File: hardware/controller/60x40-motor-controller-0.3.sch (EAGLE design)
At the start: 19 parts, among them IC1 TS432A-A3G, IC2 TS432A-A3G

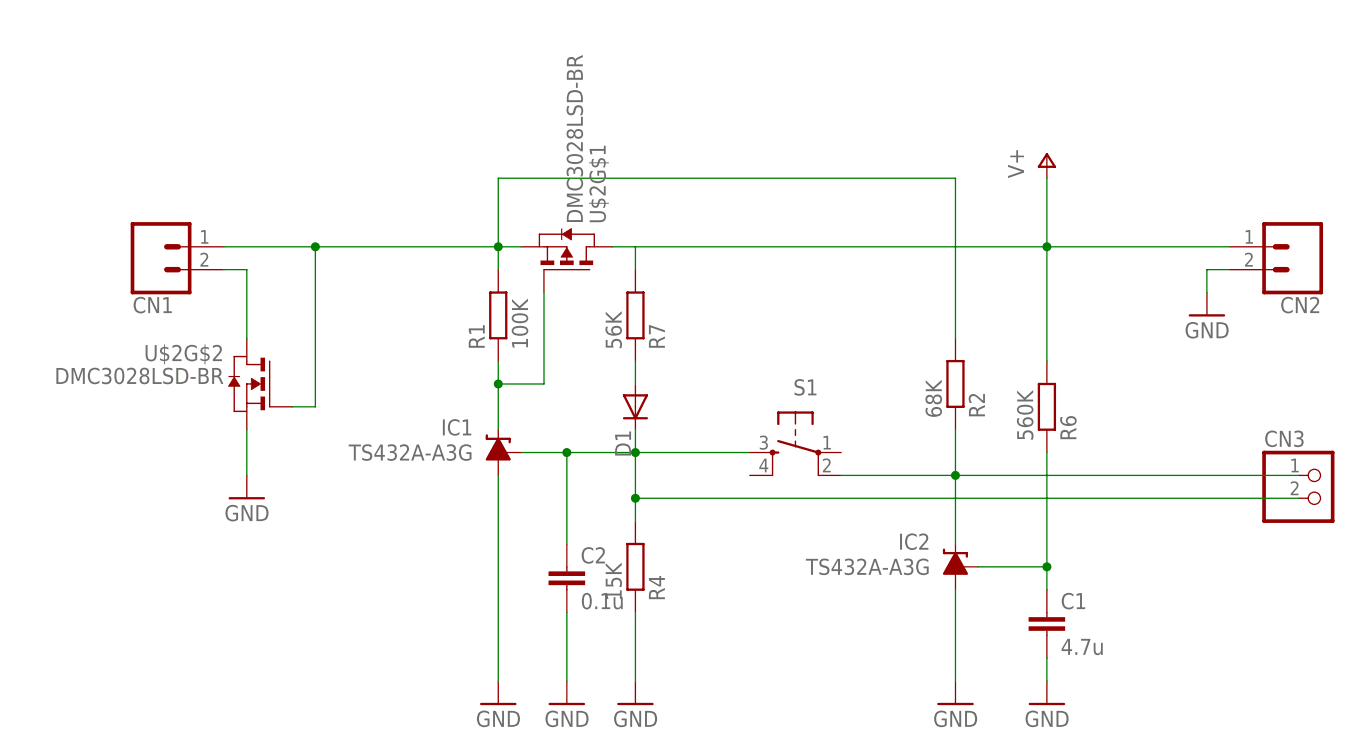
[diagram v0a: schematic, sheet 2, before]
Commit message: Lots of controller designs
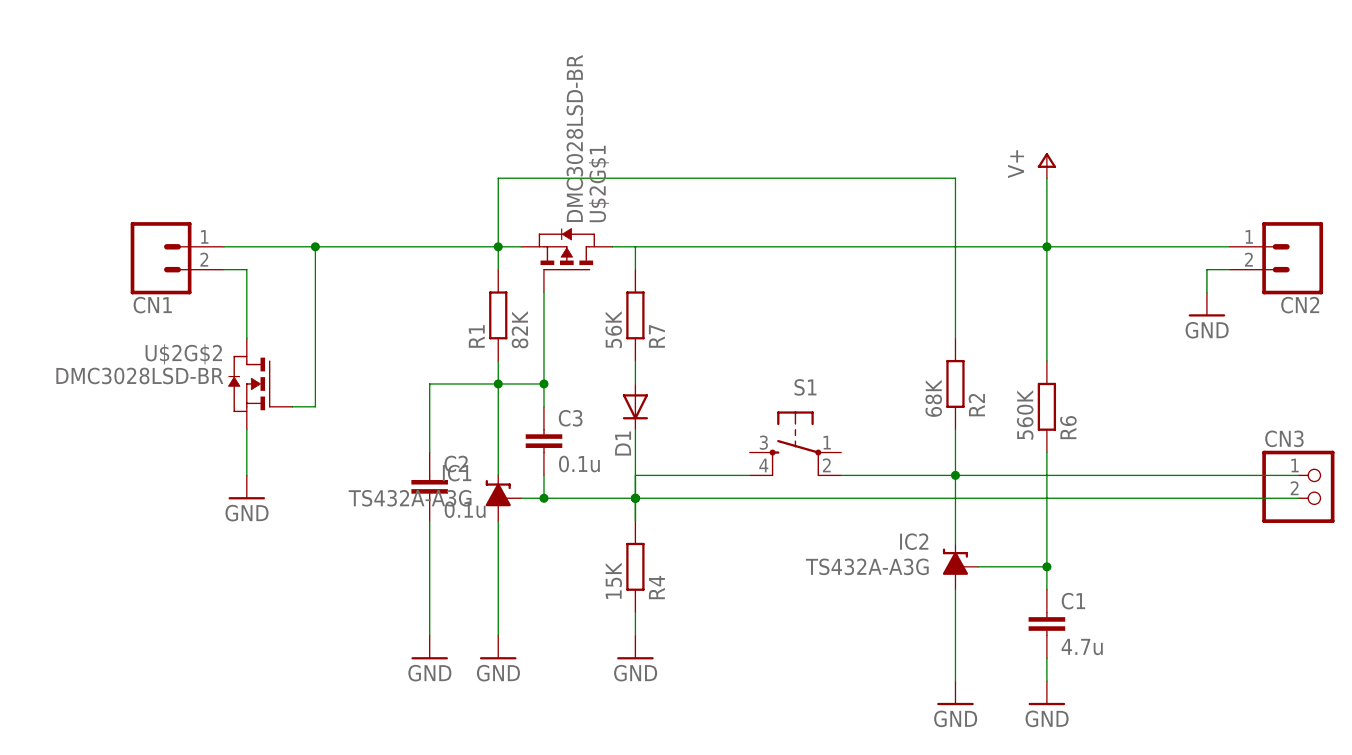
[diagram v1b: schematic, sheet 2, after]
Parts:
- added C3: 0.1u, resistor:C-EU025-024X044
- C1: device resistor:C-EU050-024X044 -> resistor:C-EU025-025X050
- D1: device diode:DIODE-D-2.5 -> diode:DIODE-D-5
- R1: value 100K -> 82K
- R2: device resistor:R-EU_0207/15 -> resistor:R-EU_0204/7
- R6: device resistor:R-EU_0204/2V -> resistor:R-EU_0207/10
- R7: device resistor:R-EU_0204/7 -> resistor:R-EU_0204/2V
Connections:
- net N$6: now also C2.1, C3.1
- net N$8: now also C3.2, S1.S1; no longer C2.1, S1.S
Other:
- moved on the sheet: C2, IC1
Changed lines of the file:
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@@
 <part name="P+1" library="supply1" deviceset="V+" device=""/>
 <part name="GND1" library="supply1" deviceset="GND" device=""/>
-<part name="R1" library="resistor" deviceset="R-EU_" device="0204/2V" value="100K"/>
+<part name="R1" library="resistor" deviceset="R-EU_" device="0204/2V" value="82K"/>
 <part name="GND2" library="supply1" deviceset="GND" device=""/>
 <part name="IC1" library="assorted" deviceset="TS432A" device="-A3G" value="TS432A-A3G"/>
 <part name="R4" library="resistor" deviceset="R-EU_" device="0204/2V" value="15K"/>
-<part name="R2" library="resistor" deviceset="R-EU_" device="0207/15" value="68K"/>
+<part name="R2" library="resistor" deviceset="R-EU_" device="0204/7" value="68K"/>
 <part name="GND3" library="supply1" deviceset="GND" device=""/>
 <part name="S1" library="assorted" deviceset="PROTO-MICRO-SWITCH" device=""/>
-<part name="C1" library="resistor" deviceset="C-EU" device="050-024X044" value="4.7u"/>
+<part name="C1" library="resistor" deviceset="C-EU" device="025-025X050" value="4.7u"/>
 <part name="GND4" library="supply1" deviceset="GND" device=""/>
-<part name="R6" library="resistor" deviceset="R-EU_" device="0204/2V" value="560K"/>
+<part name="R6" library="resistor" deviceset="R-EU_" device="0207/10" value="560K"/>
 <part name="GND5" library="supply1" deviceset="GND" device=""/>
 <part name="GND7" library="supply1" deviceset="GND" device=""/>
@@
 <part name="GND6" library="supply1" deviceset="GND" device=""/>
 <part name="IC2" library="assorted" deviceset="TS432A" device="-A3G" value="TS432A-A3G"/>
-<part name="D1" library="diode" deviceset="DIODE-" device="D-2.5"/>
+<part name="D1" library="diode" deviceset="DIODE-" device="D-5"/>
 <part name="C2" library="resistor" deviceset="C-EU" device="025-024X044" value="0.1u"/>
 <part name="GND8" library="supply1" deviceset="GND" device=""/>
 <part name="JP4" library="pinhead" deviceset="PINHD-1X4" device="/90"/>
 <part name="U$2" library="assorted" deviceset="DMC3028LSD" device="-BR"/>
-<part name="R7" library="resistor" deviceset="R-EU_" device="0204/7" value="56K"/>
+<part name="R7" library="resistor" deviceset="R-EU_" device="0204/2V" value="56K"/>
 <part name="CN3" library="pinhead" deviceset="PINHD-1X2" device="/90"/>
+<part name="C3" library="resistor" deviceset="C-EU" device="025-024X044" value="0.1u"/>
 </parts>
 <sheets>
@@
 <instances>
 <instance part="R1" gate="G$1" x="12.7" y="83.82" rot="R90"/>
-<instance part="GND2" gate="1" x="27.94" y="40.64" rot="MR0"/>
-<instance part="IC1" gate="G$1" x="12.7" y="68.58" rot="MR0"/>
+<instance part="GND2" gate="1" x="27.94" y="45.72" rot="MR0"/>
+<instance part="IC1" gate="G$1" x="12.7" y="63.5" rot="MR0"/>
 <instance part="R4" gate="G$1" x="27.94" y="55.88" rot="MR90"/>
 <instance part="R2" gate="G$1" x="63.5" y="76.2" rot="MR90"/>
@@
 <instance part="GND4" gate="1" x="73.66" y="40.64" rot="MR0"/>
 <instance part="R6" gate="G$1" x="73.66" y="73.66" rot="MR90"/>
-<instance part="GND5" gate="1" x="12.7" y="40.64" rot="MR0"/>
+<instance part="GND5" gate="1" x="12.7" y="45.72" rot="MR0"/>
 <instance part="GND7" gate="1" x="91.44" y="83.82" rot="MR0"/>
 <instance part="P+2" gate="1" x="73.66" y="101.6"/>
@@
 <instance part="IC2" gate="G$1" x="63.5" y="55.88" rot="MR0"/>
 <instance part="D1" gate="G$1" x="27.94" y="73.66" rot="MR270"/>
-<instance part="C2" gate="G$1" x="20.32" y="55.88"/>
-<instance part="GND8" gate="1" x="20.32" y="40.64" rot="MR0"/>
+<instance part="C2" gate="G$1" x="5.08" y="66.04"/>
+<instance part="GND8" gate="1" x="5.08" y="45.72" rot="MR0"/>
 <instance part="U$2" gate="G$1" x="20.32" y="91.44" rot="MR90"/>
 <instance part="U$2" gate="G$2" x="-15.24" y="76.2" rot="MR0"/>
 <instance part="R7" gate="G$1" x="27.94" y="83.82" rot="MR90"/>
 <instance part="CN3" gate="G$1" x="104.14" y="63.5"/>
+<instance part="C3" gate="G$1" x="17.78" y="71.12"/>
 </instances>
 <busses>
@@
 <pinref part="R1" gate="G$1" pin="1"/>
 <wire x1="12.7" y1="78.74" x2="12.7" y2="76.2" width="0.1524" layer="91"/>
-<wire x1="12.7" y1="76.2" x2="12.7" y2="71.12" width="0.1524" layer="91"/>
+<wire x1="12.7" y1="76.2" x2="12.7" y2="66.04" width="0.1524" layer="91"/>
 <wire x1="17.78" y1="76.2" x2="12.7" y2="76.2" width="0.1524" layer="91"/>
 <junction x="12.7" y="76.2"/>
 <pinref part="U$2" gate="G$1" pin="G"/>
+<pinref part="C3" gate="G$1" pin="1"/>
+<wire x1="17.78" y1="73.66" x2="17.78" y2="76.2" width="0.1524" layer="91"/>
+<pinref part="C2" gate="G$1" pin="1"/>
+<wire x1="12.7" y1="76.2" x2="5.08" y2="76.2" width="0.1524" layer="91"/>
+<wire x1="5.08" y1="76.2" x2="5.08" y2="68.58" width="0.1524" layer="91"/>
+<junction x="17.78" y="76.2"/>
 </segment>
 </net>
@@
 <segment>
 <pinref part="IC1" gate="G$1" pin="A"/>
-<wire x1="12.7" y1="66.04" x2="12.7" y2="43.18" width="0.1524" layer="91"/>
+<wire x1="12.7" y1="60.96" x2="12.7" y2="48.26" width="0.1524" layer="91"/>
 <pinref part="GND5" gate="1" pin="GND"/>
 </segment>
@@
 <pinref part="GND8" gate="1" pin="GND"/>
 <pinref part="C2" gate="G$1" pin="2"/>
-<wire x1="20.32" y1="43.18" x2="20.32" y2="50.8" width="0.1524" layer="91"/>
+<wire x1="5.08" y1="48.26" x2="5.08" y2="60.96" width="0.1524" layer="91"/>
 </segment>
 <segment>
 <pinref part="R4" gate="G$1" pin="1"/>
 <pinref part="GND2" gate="1" pin="GND"/>
-<wire x1="27.94" y1="50.8" x2="27.94" y2="43.18" width="0.1524" layer="91"/>
+<wire x1="27.94" y1="50.8" x2="27.94" y2="48.26" width="0.1524" layer="91"/>
 </segment>
 </net>
@@
 <segment>
 <pinref part="IC1" gate="G$1" pin="FB"/>
-<wire x1="15.24" y1="68.58" x2="20.32" y2="68.58" width="0.1524" layer="91"/>
-<pinref part="C2" gate="G$1" pin="1"/>
-<wire x1="20.32" y1="58.42" x2="20.32" y2="68.58" width="0.1524" layer="91"/>
+<wire x1="15.24" y1="63.5" x2="17.78" y2="63.5" width="0.1524" layer="91"/>
 <pinref part="R4" gate="G$1" pin="2"/>
 <wire x1="27.94" y1="60.96" x2="27.94" y2="63.5" width="0.1524" layer="91"/>
-<wire x1="27.94" y1="63.5" x2="27.94" y2="68.58" width="0.1524" layer="91"/>
-<wire x1="20.32" y1="68.58" x2="27.94" y2="68.58" width="0.1524" layer="91"/>
-<junction x="20.32" y="68.58"/>
+<wire x1="17.78" y1="63.5" x2="27.94" y2="63.5" width="0.1524" layer="91"/>
 <pinref part="D1" gate="G$1" pin="C"/>
-<wire x1="27.94" y1="71.12" x2="27.94" y2="68.58" width="0.1524" layer="91"/>
-<pinref part="S1" gate="1" pin="S"/>
-<wire x1="40.64" y1="68.58" x2="27.94" y2="68.58" width="0.1524" layer="91"/>
-<junction x="27.94" y="68.58"/>
+<wire x1="27.94" y1="71.12" x2="27.94" y2="63.5" width="0.1524" layer="91"/>
+<junction x="27.94" y="63.5"/>
 <pinref part="CN3" gate="G$1" pin="2"/>
 <wire x1="101.6" y1="63.5" x2="27.94" y2="63.5" width="0.1524" layer="91"/>
 <junction x="27.94" y="63.5"/>
-</segment>
-</net>
+<pinref part="S1" gate="1" pin="S1"/>
+<wire x1="40.64" y1="66.04" x2="27.94" y2="66.04" width="0.1524" layer="91"/>
+<wire x1="27.94" y1="66.04" x2="27.94" y2="60.96" width="0.1524" layer="91"/>
+<pinref part="C3" gate="G$1" pin="2"/>
+<wire x1="17.78" y1="66.04" x2="17.78" y2="63.5" width="0.1524" layer="91"/>
+<junction x="17.78" y="63.5"/>
+</segment>
+</net>
